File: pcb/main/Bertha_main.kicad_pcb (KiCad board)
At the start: 2 copper layers, 100 x 87 mm, 159 parts, among them IC1 SST26VF064B-104V, IC2 DRV8811, J1 RJ12, J10 SJ, J11 SJ, J12 AudioJack3_SwitchTR, J2 Conn_Coaxial_Power, J3 Conn_02x03_Odd_Even, J4 RJ12, J5 AudioJack3_SwitchTR, J6 SJ, J7 Conn_01x01, J8 Conn_01x01, J9 SJ, Q1 ZXMS6004, Q2 ZXMS6004, Q3 IPB80N03S4L-03, Q4 TRANSISTOR_PNPMMBT4403, Q5 ZXMS6004, Q6 ZXMS6004, Q7 ZXMS6004, Q8 ZXMS6004, U1 DS18B20, U2 ATMEGA32U4-AU, U3 ACT4088, U4 HX711, X1 MINI-USB-SCHIELD-32005-201, Y1 Crystal

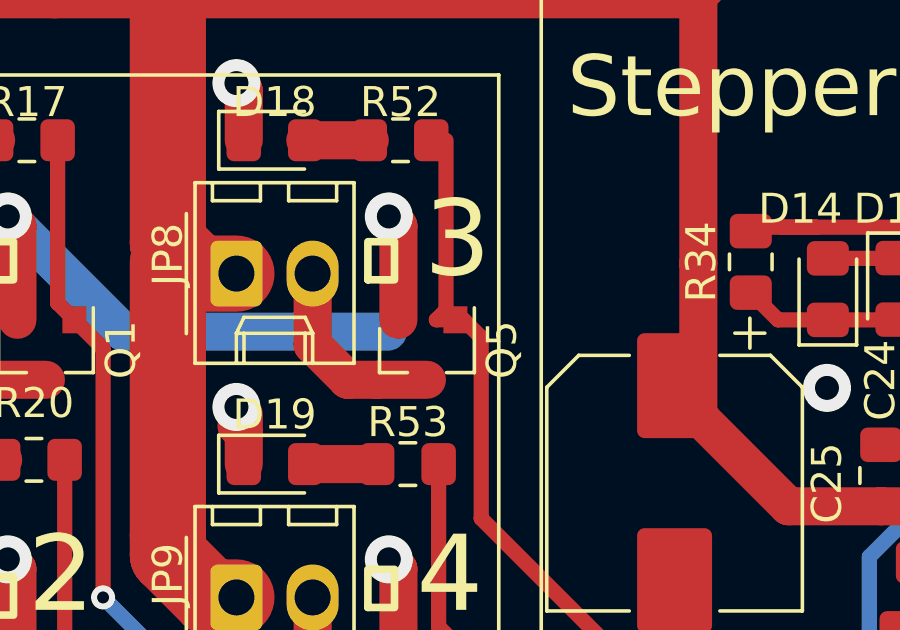
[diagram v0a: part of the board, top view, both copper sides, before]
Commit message: docs(BOM): iBOM.html updated
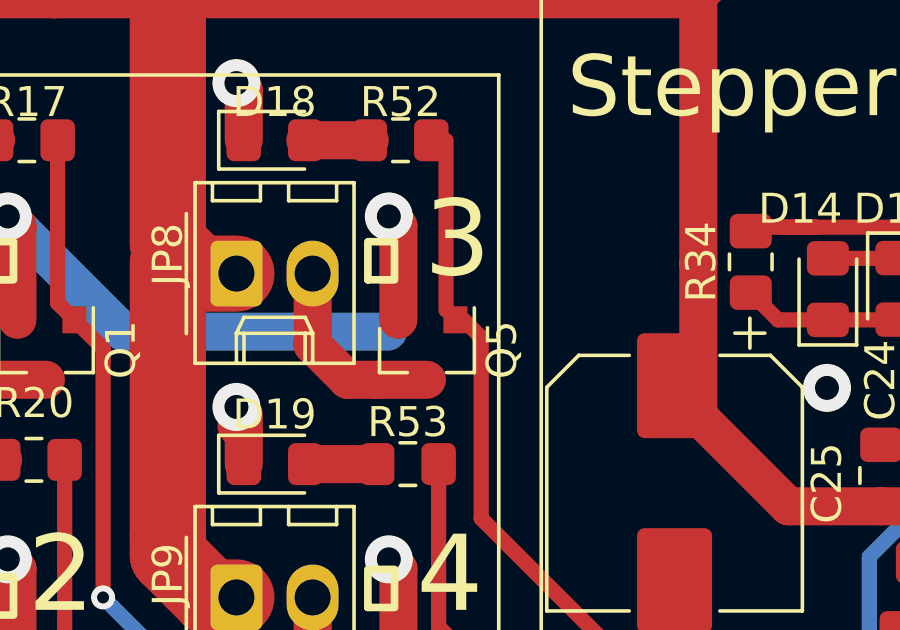
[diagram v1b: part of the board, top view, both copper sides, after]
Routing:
- net A6: track 43.1 -> 41.8 mm
